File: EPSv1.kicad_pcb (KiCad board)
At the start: 4 copper layers, 100 x 100 mm, 150 parts, among them J1 1053091102, J2 1053091102, J3 1053091102, J4 Conn_01x05_Pin, Q1 AO3400A, Q2 AO3400A, Q3 AO3400A, Q4 AO3400A, Q5 AP25P06K, U1 MCP9700AT-E/TT, U10 C3235556 (M66200DRLR), U11 STM32L432KCUx, U12 C3235556 (M66200DRLR), U13 C3235556 (M66200DRLR), U14 1.5uF 2.9A, U15 TPS63070RNMR, U16 1.5uF 2.9A, U17 TPS63070RNMR, U18 20m 1206, U19 INA199A1DCKR, U2 MCP9700AT-E/TT, U20 20m 1206, U21 INA199A1DCKR, U22 20m 1206, U23 INA199A1DCKR, U24 1.5uF 2.9A, U25 TPS63070RNMR, U26 1.5uF 2.9A, U3 BQ29700DSER, U4 BQ29700DSER, U5 MCP73831T-2ACI/OT, U6 MCP73831T-2ACI/OT, U7 C3235556 (M66200DRLR), U8 C3235556 (M66200DRLR), U9 C3235556 (M66200DRLR)

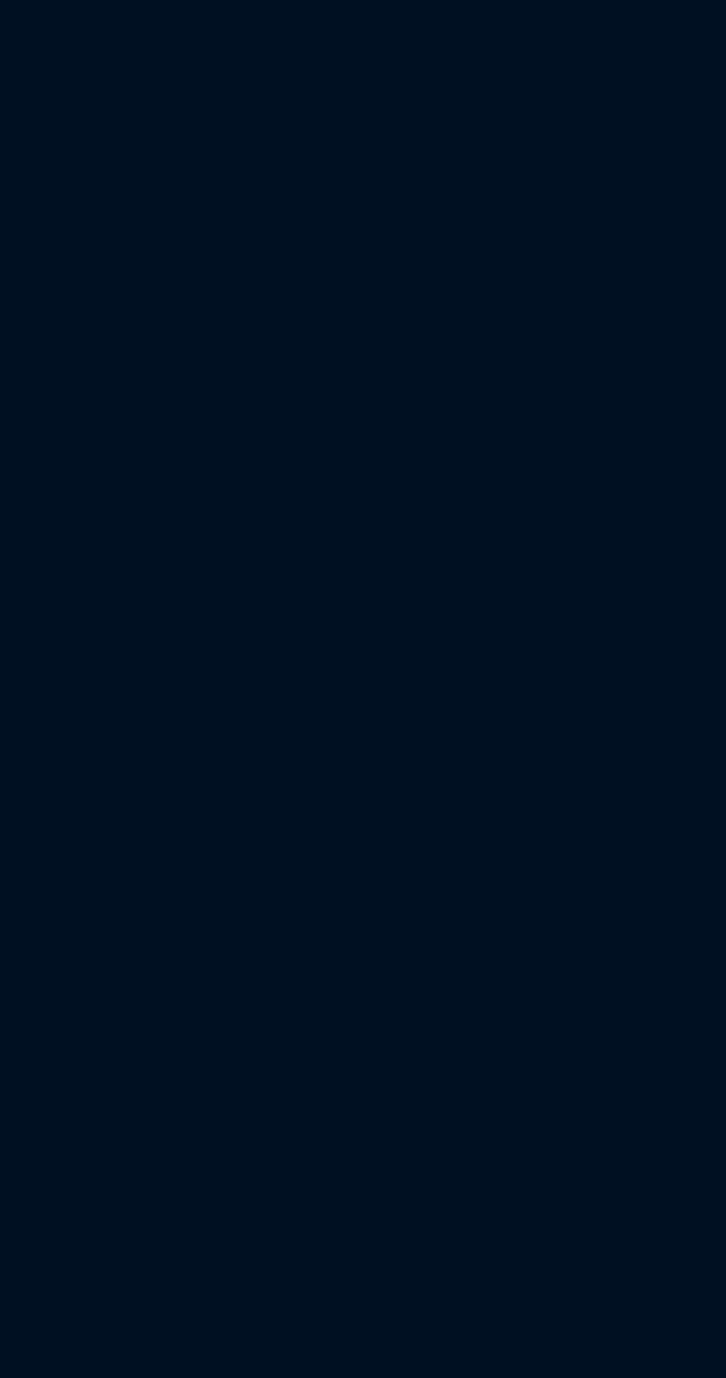
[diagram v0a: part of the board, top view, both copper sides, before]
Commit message: testing
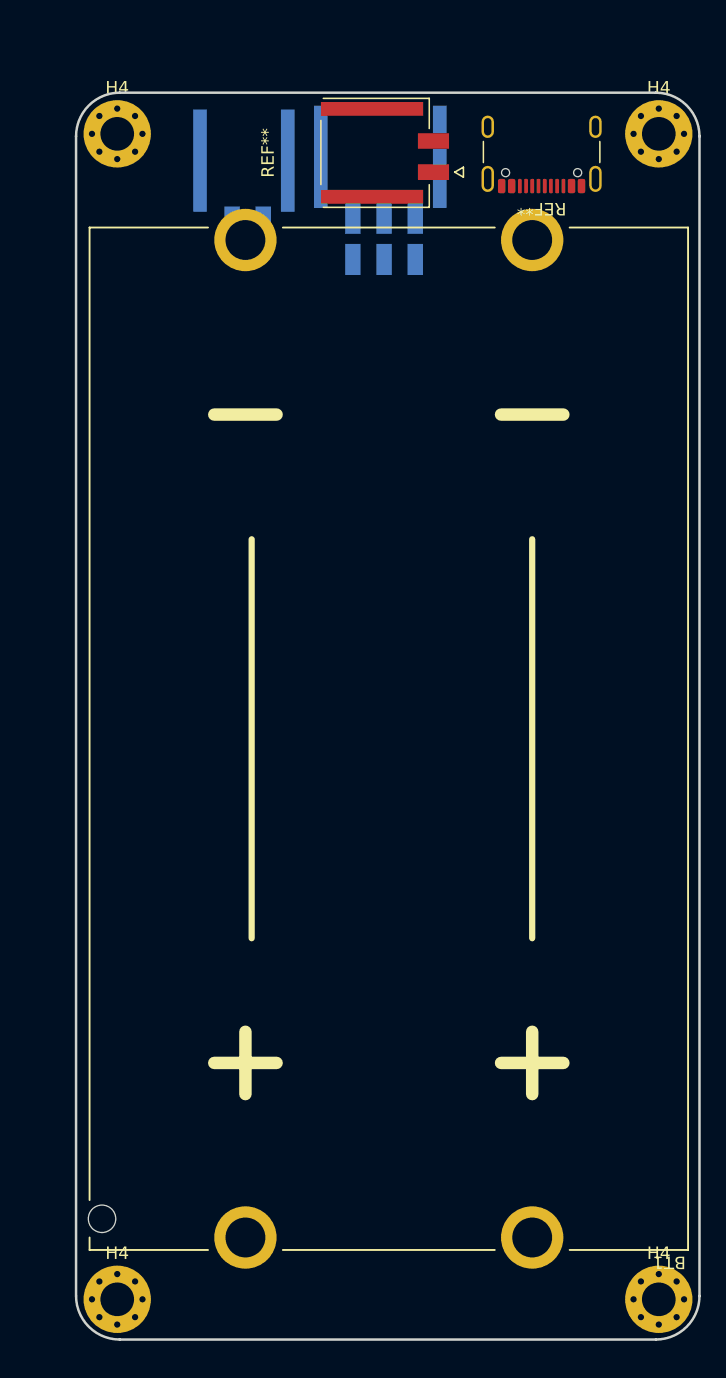
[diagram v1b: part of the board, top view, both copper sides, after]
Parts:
- added BT1: 2P 21700 Cell Holder, Rocketry_Manual:PA21700x2-THM_Parallel, F.Cu at (213.4, 124.3)
- added H4: MountingHole_Pad, MountingHole:MountingHole_2.7mm_M2.5_Pad_Via, F.Cu at (211.1, 34.8)
- added H4: MountingHole_Pad, MountingHole:MountingHole_2.7mm_M2.5_Pad_Via, F.Cu at (211.1, 128.3)
- added H4: MountingHole_Pad, MountingHole:MountingHole_2.7mm_M2.5_Pad_Via, F.Cu at (167.6, 34.8)
- added H4: MountingHole_Pad, MountingHole:MountingHole_2.7mm_M2.5_Pad_Via, F.Cu at (167.6, 128.3)
- added REF**: MOLEX_1054301102, Rocketry_Manual:1054301102, F.Cu at (189.2, 36.3)
- added REF**: USB_C_Receptacle_GCT_USB4105-xx-A_16P_TopMnt_Horizontal, Connector_USB:USB_C_Receptacle_GCT_USB4105-xx-A_16P_TopMnt_Horizontal, F.Cu at (201.7, 35.3)
- added REF**: MOLEX_1054301102, Rocketry_Manual:1054301102, B.Cu at (177.8, 38.1)
- added REF**: MOLEX_1054051106, Rocketry_Manual:1054051106, B.Cu at (188.7, 38.4)
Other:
- board size 100 x 100 mm -> 196 x 104.1 mm
